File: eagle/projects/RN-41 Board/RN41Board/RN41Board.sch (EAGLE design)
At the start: 18 parts, among them Q1 MOSFET-NCHANNELSMD, U1 BLUETOOTH-RN41, U3 3.3V

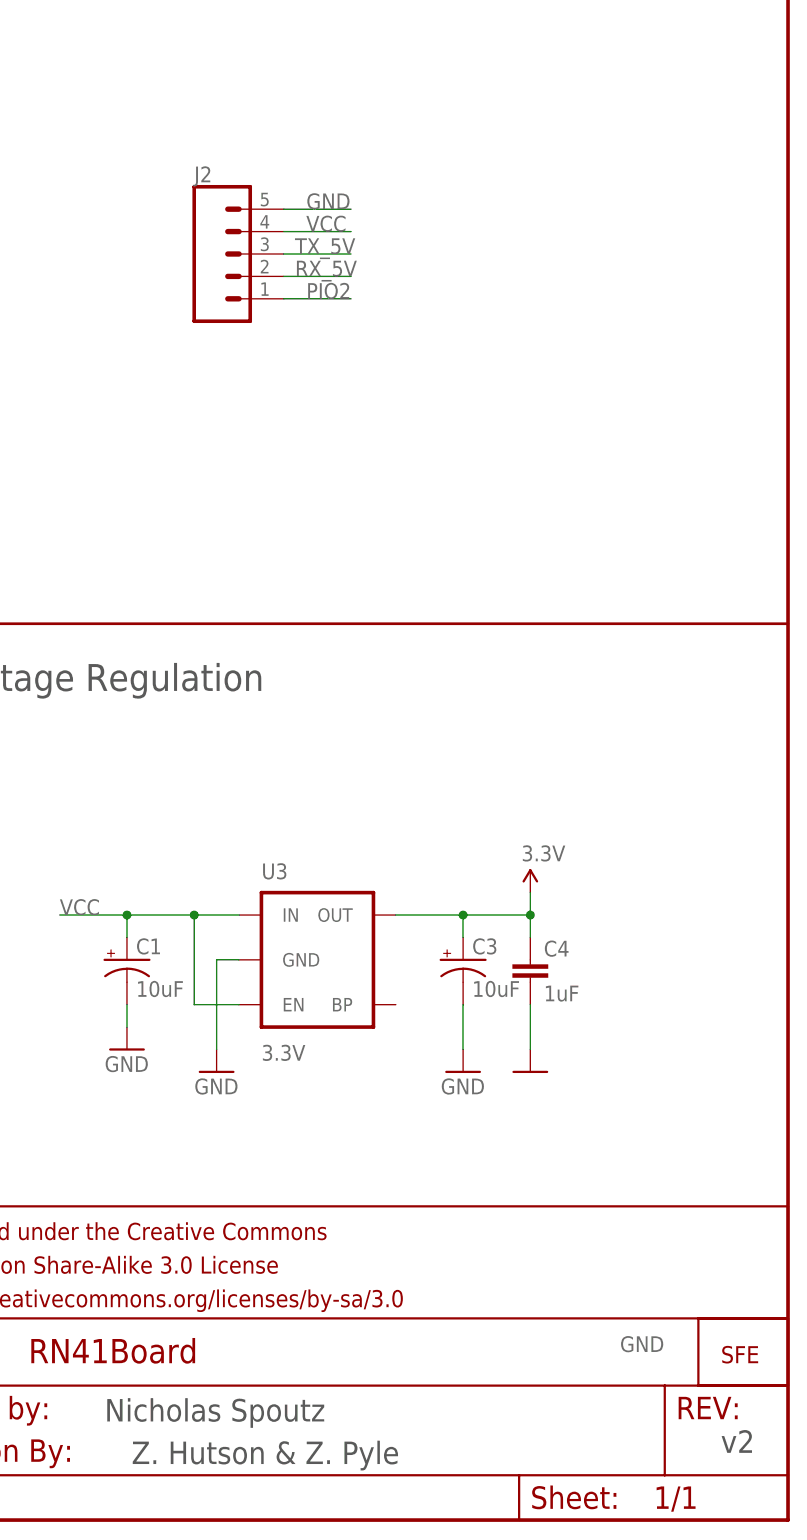
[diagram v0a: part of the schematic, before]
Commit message: RN41Board UPDATE
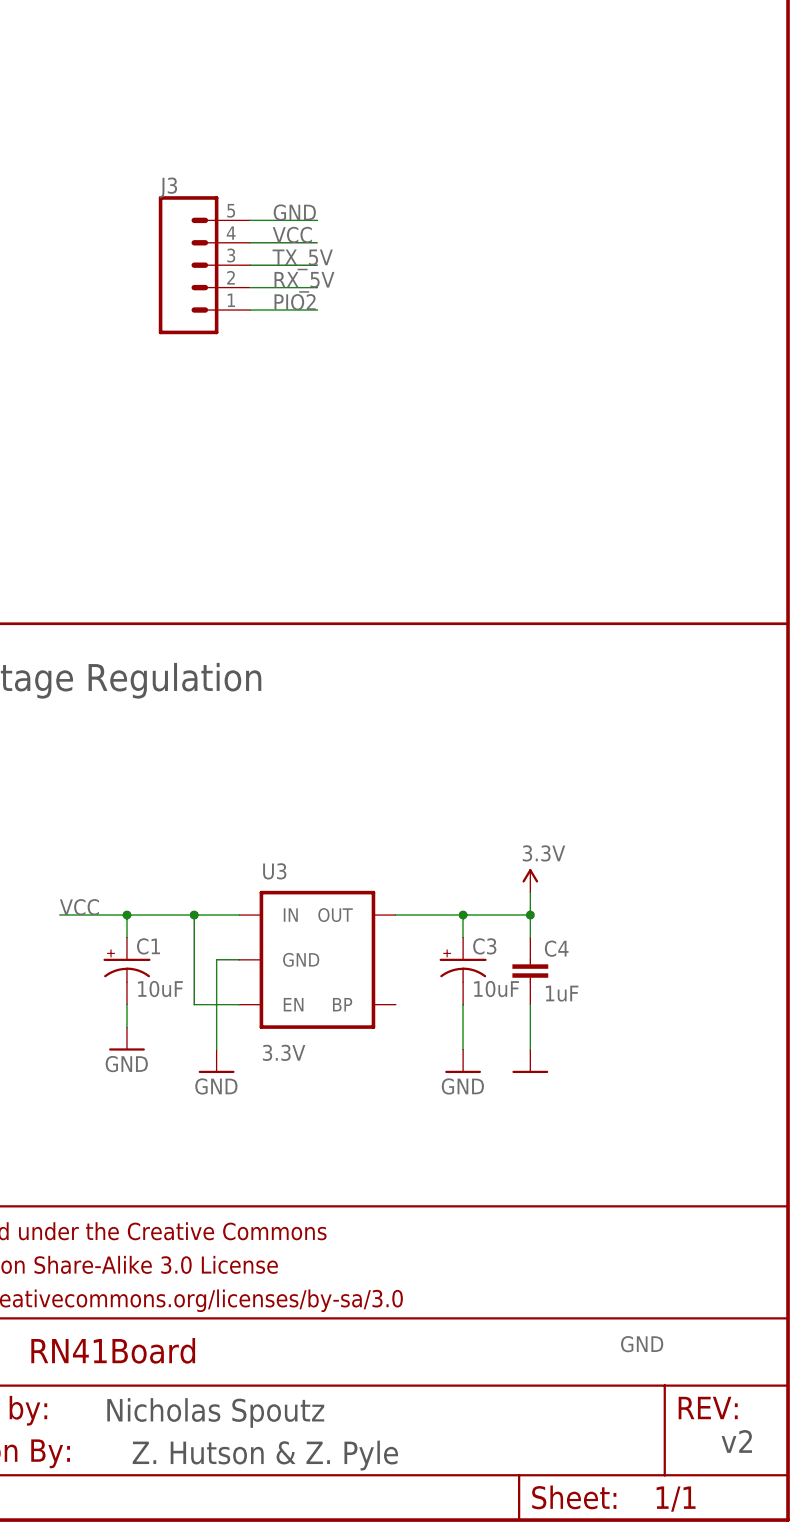
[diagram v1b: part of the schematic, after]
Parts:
- removed J2: (no value), SparkFun-Connectors:CONN_05JST
- removed U$1: LOGO-SFENEW, SparkFun:LOGO-SFENEW
- added J3: (no value), SparkFun-Connectors:CONN_05
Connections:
- net GND: now also J3.5; no longer J2.5
- net PIO2: now also J3.1; no longer J2.1
- net RX_5V: now also J3.2; no longer J2.2
- net TX_5V: now also J3.3; no longer J2.3
- net VCC: now also J3.4; no longer J2.4
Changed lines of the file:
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@@
 <setting verticaltext="up"/>
 </settings>
-<grid distance="0.05" unitdist="inch" unit="inch" style="lines" multiple="1" display="yes" altdistance="0.01" altunitdist="inch" altunit="inch"/>
+<grid distance="0.1" unitdist="inch" unit="inch" style="lines" multiple="1" display="no" altdistance="0.01" altunitdist="inch" altunit="inch"/>
 <layers>
 <layer number="1" name="Top" color="4" fill="1" visible="no" active="no"/>
@@
 <part name="U3" library="SparkFun" deviceset="V_REG_LDO" device="SMD" value="3.3V"/>
 <part name="R1" library="SparkFun" deviceset="RESISTOR" device="0603-RES" value="330"/>
-<part name="U$1" library="SparkFun" deviceset="LOGO-SFE" device="NEW"/>
 <part name="GND2" library="SparkFun" deviceset="GND" device=""/>
 <part name="GND4" library="SparkFun" deviceset="GND" device=""/>
@@
 <part name="GND8" library="SparkFun" deviceset="GND" device=""/>
 <part name="U$2" library="SparkFun-Aesthetics" deviceset="REVISION" device=""/>
-<part name="J2" library="SparkFun-Connectors" deviceset="CONN_05" device="JST"/>
+<part name="J3" library="SparkFun-Connectors" deviceset="CONN_05" device=""/>
 </parts>
 <sheets>
@@
 <attribute name="VALUE" x="98.298" y="24.13" size="1.778" layer="96" rot="R270"/>
 </instance>
-<instance part="U$1" gate="G$1" x="241.3" y="17.78" smashed="yes"/>
 <instance part="GND2" gate="1" x="101.6" y="10.16" smashed="yes">
 <attribute name="VALUE" x="99.06" y="7.62" size="1.778" layer="96"/>
@@
 </instance>
 <instance part="U$2" gate="G$1" x="148.59" y="6.604" smashed="yes"/>
-<instance part="J2" gate="G$1" x="184.15" y="143.51" smashed="yes">
-<attribute name="VALUE" x="181.61" y="133.604" size="1.778" layer="96" font="vector"/>
-<attribute name="NAME" x="181.61" y="151.638" size="1.778" layer="95" font="vector"/>
+<instance part="J3" gate="G$1" x="180.34" y="142.24" smashed="yes">
+<attribute name="VALUE" x="177.8" y="132.334" size="1.778" layer="96" font="vector"/>
+<attribute name="NAME" x="177.8" y="150.368" size="1.778" layer="95" font="vector"/>
 </instance>
 </instances>
@@
 </segment>
 <segment>
-<pinref part="J2" gate="G$1" pin="5"/>
-<wire x1="191.77" y1="148.59" x2="199.39" y2="148.59" width="0.1524" layer="91"/>
-<label x="194.31" y="148.59" size="1.778" layer="95"/>
+<pinref part="J3" gate="G$1" pin="5"/>
+<wire x1="187.96" y1="147.32" x2="195.58" y2="147.32" width="0.1524" layer="91"/>
+<label x="190.5" y="147.32" size="1.778" layer="95"/>
 </segment>
 </net>
@@
 </segment>
 <segment>
-<pinref part="J2" gate="G$1" pin="3"/>
-<wire x1="191.77" y1="143.51" x2="199.39" y2="143.51" width="0.1524" layer="91"/>
-<label x="193.04" y="143.51" size="1.778" layer="95"/>
+<pinref part="J3" gate="G$1" pin="3"/>
+<wire x1="187.96" y1="142.24" x2="195.58" y2="142.24" width="0.1524" layer="91"/>
+<label x="190.5" y="142.24" size="1.778" layer="95"/>
 </segment>
 </net>
@@
 </segment>
 <segment>
-<pinref part="J2" gate="G$1" pin="2"/>
-<wire x1="191.77" y1="140.97" x2="199.39" y2="140.97" width="0.1524" layer="91"/>
-<label x="193.04" y="140.97" size="1.778" layer="95"/>
+<pinref part="J3" gate="G$1" pin="2"/>
+<wire x1="187.96" y1="139.7" x2="195.58" y2="139.7" width="0.1524" layer="91"/>
+<label x="190.5" y="139.7" size="1.778" layer="95"/>
 </segment>
 </net>
@@
 </segment>
 <segment>
-<pinref part="J2" gate="G$1" pin="4"/>
-<wire x1="191.77" y1="146.05" x2="199.39" y2="146.05" width="0.1524" layer="91"/>
-<label x="194.31" y="146.05" size="1.778" layer="95"/>
+<pinref part="J3" gate="G$1" pin="4"/>
+<wire x1="187.96" y1="144.78" x2="195.58" y2="144.78" width="0.1524" layer="91"/>
+<label x="190.5" y="144.78" size="1.778" layer="95"/>
 </segment>
 </net>
@@
 </segment>
 <segment>
-<pinref part="J2" gate="G$1" pin="1"/>
-<wire x1="191.77" y1="138.43" x2="199.39" y2="138.43" width="0.1524" layer="91"/>
-<label x="194.31" y="138.43" size="1.778" layer="95"/>
-</segment>
-</net>
+<pinref part="J3" gate="G$1" pin="1"/>
+<wire x1="187.96" y1="137.16" x2="195.58" y2="137.16" width="0.1524" layer="91"/>
+<label x="190.5" y="137.16" size="1.778" layer="95"/>
+</segment>
+</net>
